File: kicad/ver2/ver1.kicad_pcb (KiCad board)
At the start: 2 copper layers, 74 parts, among them SW1 SW_PUSH, SW10 SW_PUSH, SW11 SW_PUSH, SW12 SW_PUSH, SW13 SW_PUSH, SW14 SW_PUSH, SW15 SW_PUSH, SW16 SW_PUSH, SW17 SW_PUSH, SW18 SW_PUSH, SW19 SW_PUSH, SW2 SW_PUSH, SW20 SW_PUSH, SW21 SW_PUSH, SW22 SW_PUSH, SW23 SW_PUSH, SW24 SW_PUSH, SW25 SW_PUSH, SW26 SW_PUSH, SW27 SW_PUSH, SW28 SW_PUSH, SW29 SW_PUSH, SW3 SW_PUSH, SW30 SW_PUSH, SW31 SW_PUSH, SW32 SW_PUSH, SW33 SW_PUSH, SW34 SW_PUSH, SW35 SW_PUSH, SW36 SW_PUSH, SW37 SW_PUSH, SW4 SW_PUSH, SW5 SW_PUSH, SW6 SW_PUSH, SW7 SW_PUSH, SW8 SW_PUSH, SW9 SW_PUSH, U1 ProMicro_r

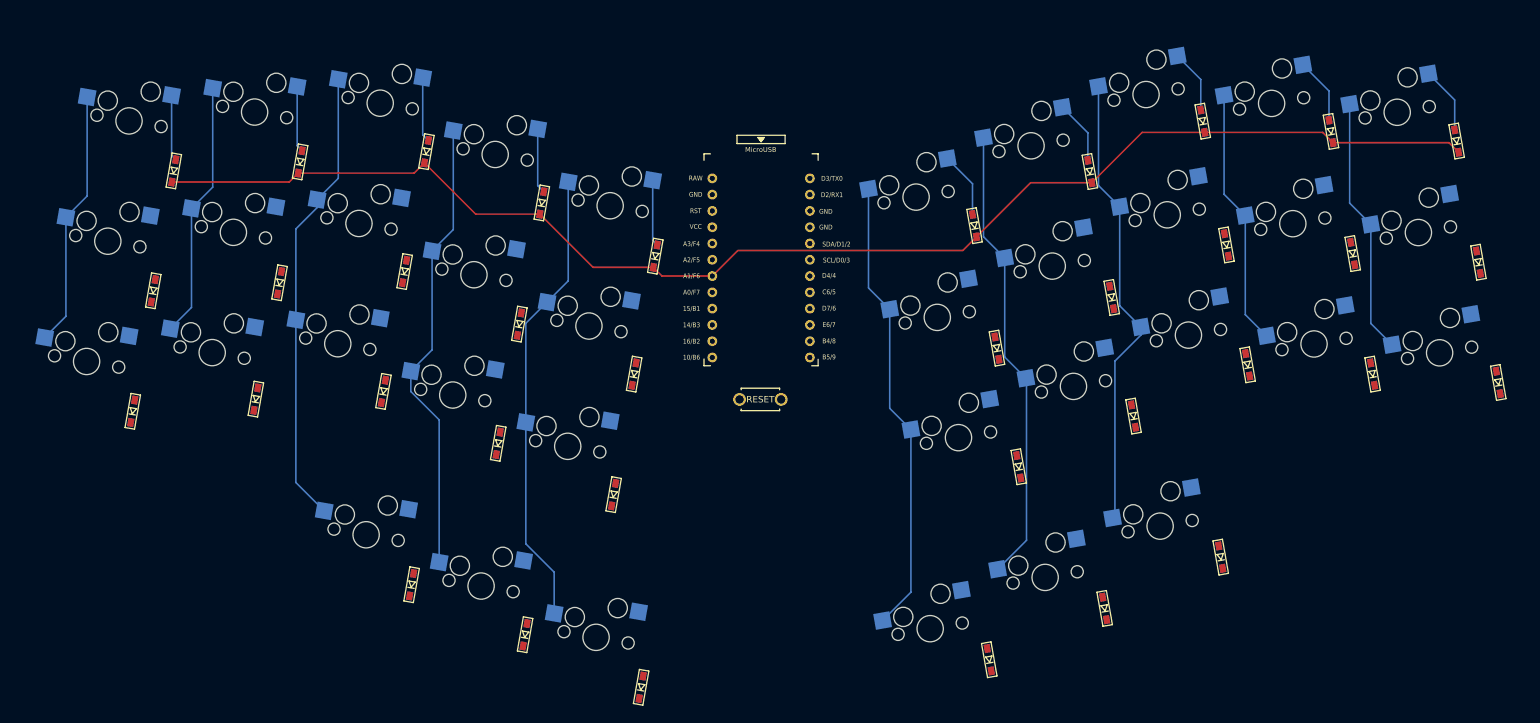
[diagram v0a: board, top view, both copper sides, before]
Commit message: add ver2
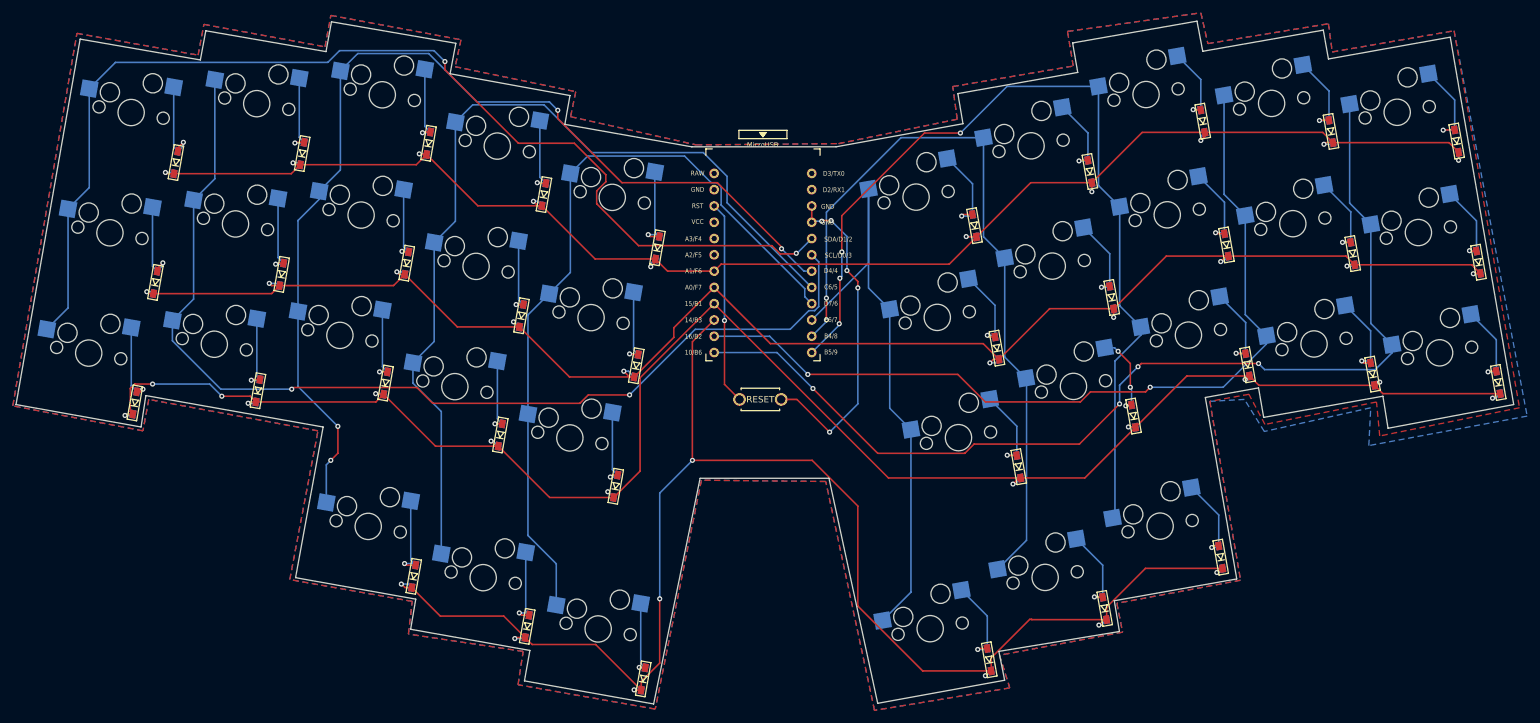
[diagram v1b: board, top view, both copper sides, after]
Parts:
- moved D12 1.35 mm to (63.4, 75.7)
- moved D22 1.35 mm to (59.7, 93.8)
- moved D32 1.35 mm to (101.7, 130.6)
- moved D33 1.35 mm to (119.8, 138.8)
- moved D5 1.35 mm to (122.0, 71.5)
- moved SW14 1.35 mm to (93.8, 74.4)
- moved SW15 1.35 mm to (111.7, 82.4)
- moved SW21 1.35 mm to (33.3, 88.0)
- moved SW24 1.35 mm to (90.4, 93.2)
- moved SW25 1.35 mm to (108.4, 101.2)
- moved SW31 1.35 mm to (76.9, 115.0)
- moved SW33 1.35 mm to (112.8, 131.0)
- moved D1 1.35 mm to (46.9, 58.2)
- moved D2 1.35 mm to (66.6, 56.8)
- moved D3 1.35 mm to (86.3, 55.2)
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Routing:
- net Row3: track 0.00 -> 292.1 mm, vias 0 -> 12
- net Row2: track 0.00 -> 263.0 mm, vias 0 -> 10
- net Row4: track 0.00 -> 236.6 mm, vias 0 -> 8
- net Column1: track 40.3 -> 174.9 mm, vias 0 -> 2
- net Column2: track 40.3 -> 163.3 mm, vias 0 -> 2
- net Column10: track 40.3 -> 162.8 mm, vias 0 -> 4
- net Column9: track 40.3 -> 135.7 mm, vias 0 -> 2
- net Column3: track 71.9 -> 163.0 mm, vias 0 -> 4
- net Column8: track 71.9 -> 143.6 mm, vias 0 -> 4
- net Column4: track 71.9 -> 142.8 mm
- net GND: track 0.00 -> 52.3 mm, vias 0 -> 5
- net Column5: track 71.9 -> 122.6 mm
- net Column7: track 72.0 -> 121.6 mm, vias 0 -> 2
- net Net-(U1-RST): track 0.00 -> 31.8 mm, vias 0 -> 1
- net Row1: track 219.8 -> 247.9 mm, vias 0 -> 10
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- added copper zone on B.Cu, net (none)
- added copper zone on F.Cu, net GND
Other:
- board outline added: 233.6 x 106.5 mm
